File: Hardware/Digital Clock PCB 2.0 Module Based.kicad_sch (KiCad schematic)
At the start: 16 parts, among them J1 USB_C_Receptacle_USB2.0, J2 Conn_01x04, J3 Conn_01x04, SW1 SW_Push, SW2 SW_Push, U1 ESP32-S2-SOLO-2, U2 AMS1117-3.3

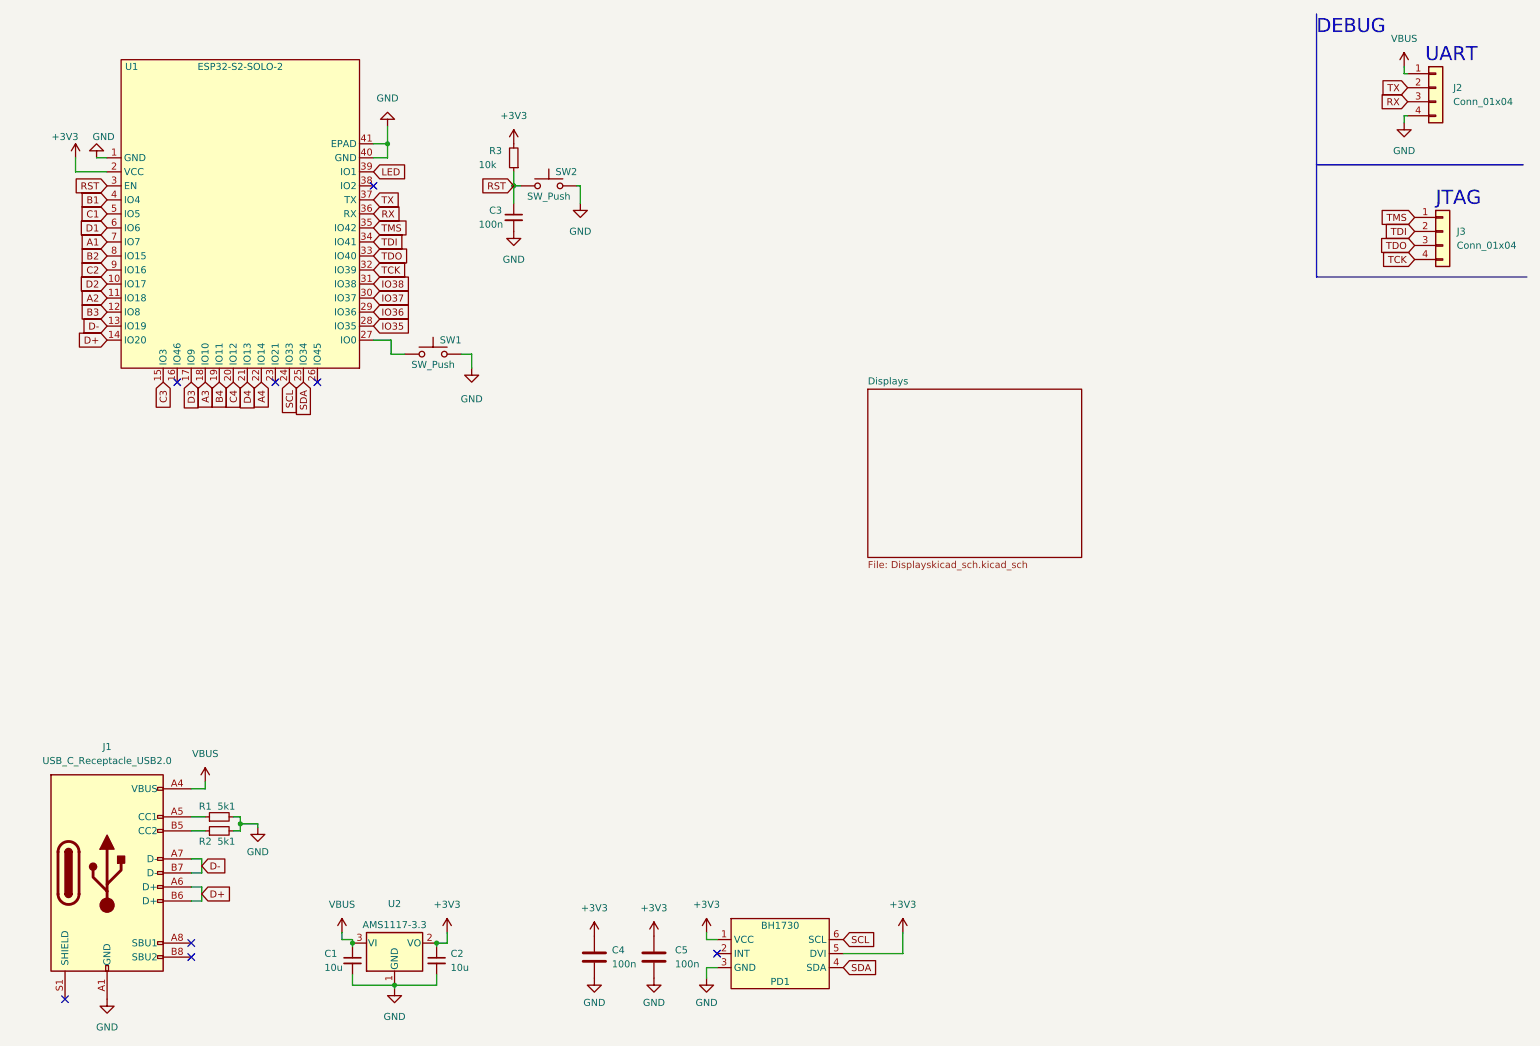
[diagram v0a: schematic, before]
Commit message: Final revision for this run
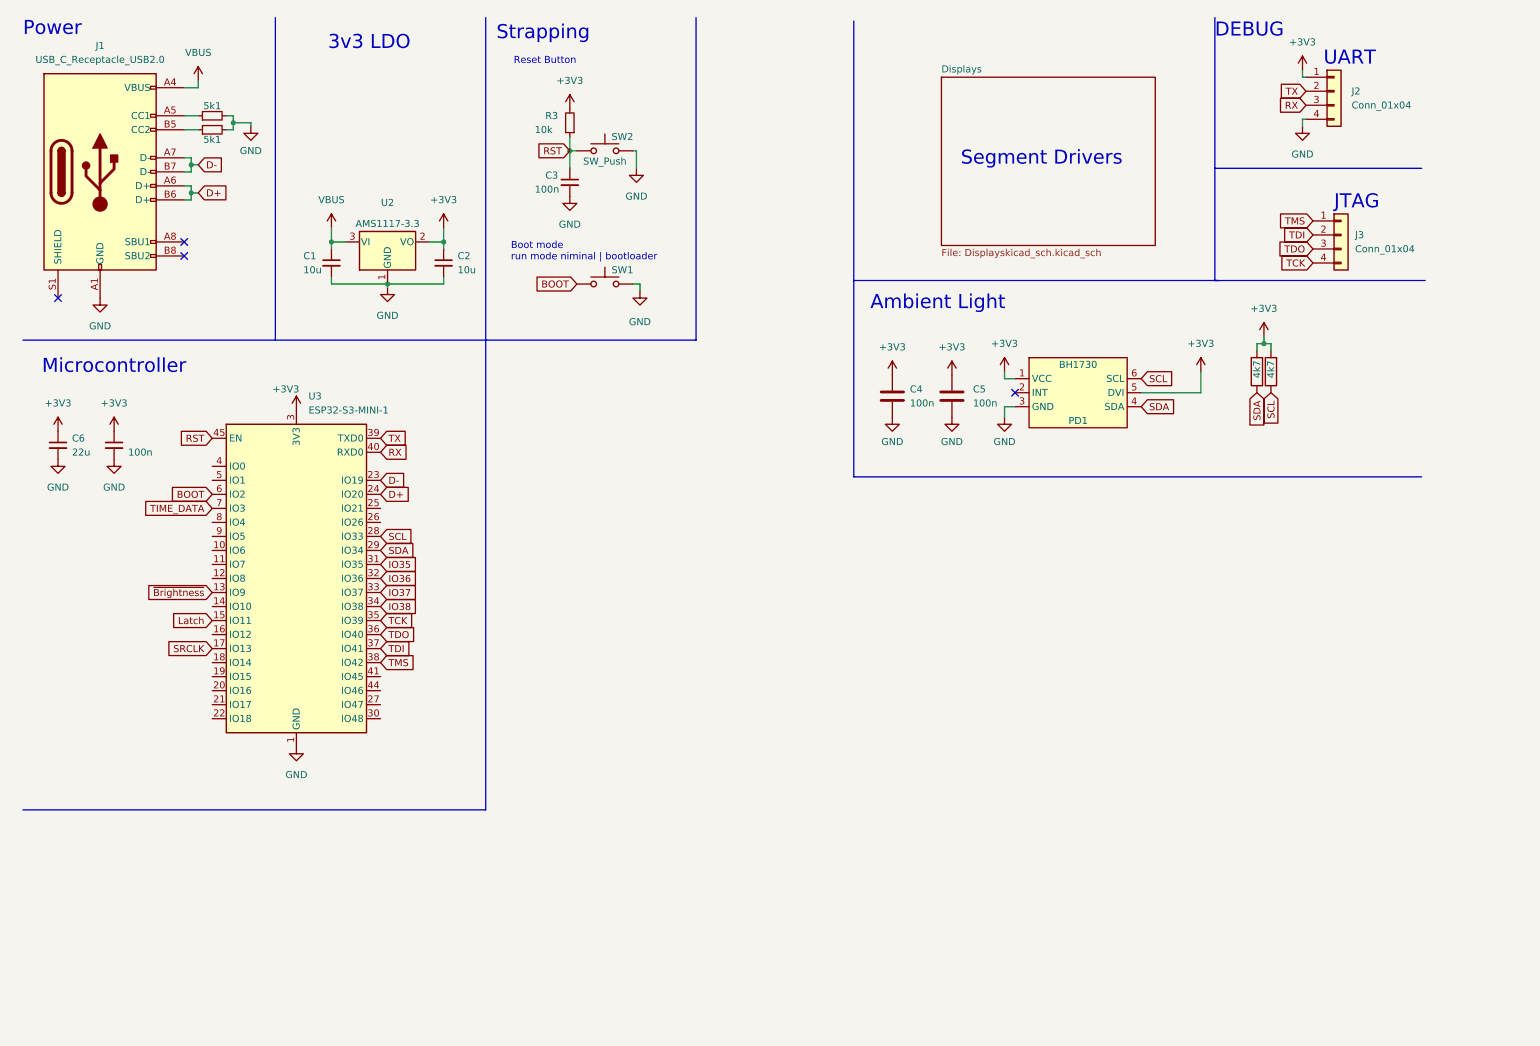
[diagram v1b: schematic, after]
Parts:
- removed U1: ESP32-S2-SOLO-2, RF_Module:ESP32-S3-WROOM-1, symbol S2 Solo:ESP32-S2-SOLO-2
- added C6: 22u, Capacitor_SMD:C_0603_1608Metric, symbol Device:C_Small
- added C7: 100n, Capacitor_SMD:C_0603_1608Metric, symbol Device:C_Small
- added R7, R8: 4k7, Resistor_SMD:R_0603_1608Metric, symbol Device:R
- added U3: ESP32-S3-MINI-1, RF_Module:ESP32-S2-MINI-1, symbol RF_Module:ESP32-S3-MINI-1
- SW1, SW2: footprint Ian's Custom Components:5.2mm_Tactile_Push_Button -> Button_Switch_SMD:SW_SPST_SKQG_WithStem
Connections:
- net +3V3: now also J2.1 (Pin_1), C6.1, C7.1, R7.2, R8.2, U3.3 (3V3)
- net D+: now also U3.24 (IO20)
- net D-: now also U3.23 (IO19)
- net GND: now also C6.2, C7.2, U3.1 (GND), U3.2 (GND), U3.42 (GND), U3.43 (GND), U3.46 (GND), U3.47 (GND), U3.48 (GND), U3.49 (GND), U3.50 (GND), U3.51 (GND), U3.52 (GND), U3.53 (GND), U3.54 (GND), U3.55 (GND), U3.56 (GND), U3.57 (GND), U3.58 (GND), U3.59 (GND), U3.60 (GND), U3.61 (GND), U3.62 (GND), U3.63 (GND), U3.64 (GND), U3.65 (GND)
- net IO35: now also U3.31 (IO35)
- net IO36: now also U3.32 (IO36)
- net IO37: now also U3.33 (IO37)
- net IO38: now also U3.34 (IO38)
- net RST: now also U3.45 (EN)
- net RX: now also U3.40 (RXD0)
- net SCL: now also R7.1, U3.28 (IO33)
- net SDA: now also R8.1, U3.29 (IO34)
- net TCK: now also U3.35 (IO39)
- net TDI: now also U3.37 (IO41)
- net TDO: now also U3.36 (IO40)
- net TMS: now also U3.38 (IO42)
- net TX: now also U3.39 (TXD0)
- net VBUS: no longer J2.1 (Pin_1)
- net BOOT: now reaches SW1.1
- net BOOT: now also U3.6 (IO2)
- new net Latch: U3.15 (IO11)
- new net SRCLK: U3.17 (IO13)
- new net TIME_DATA: U3.7 (IO3)
- new net ~{Brightness}: U3.13 (IO9)
- no-connect marks 8 -> 4
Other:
- note added: "3v3 LDO"
- note added: "Ambient Light"
- note added: "Boot mode run mode niminal | bootloader"
- note added: "Microcontroller"
- note added: "Power"
- note added: "Reset Button"
- note added: "Segment Drivers"
- note added: "Strapping"
- company: (none) -> Casual Coders LLC
- title: (none) -> RedShift
- moved on the sheet: C1, C2, C3, C4, C5, J1, J2, J3, PD1, R3, SW1, SW2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
